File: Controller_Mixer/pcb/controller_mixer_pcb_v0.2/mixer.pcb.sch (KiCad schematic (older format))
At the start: 78 parts, among them J1 Conn_01x03, J10 Conn_01x02, J11 Conn_01x02, J12 Conn_01x02, J13 Conn_01x02, J14 Conn_01x02, J15 Conn_01x02, J16 Conn_01x02, J2 Conn_01x03, J3 Conn_01x03, J4 Conn_01x03, J41 Conn_01x04, J42 Conn_01x04, J43 Conn_01x03, J44 Conn_01x02, J45 Conn_01x02, J46 Conn_01x02, J47 Conn_01x02, J48 Conn_01x02, J49 Conn_01x02, J5 Conn_01x03, J50 Conn_01x02, J51 Conn_01x02, J52 Conn_01x02, J53 Conn_01x02, J54 Conn_01x05, J55 Conn_01x05, J56 Conn_01x05, J57 Conn_01x05, J58 Conn_01x05, J59 Conn_01x05, J6 Conn_01x03, J7 Conn_01x03, J71 Conn_01x03, J72 Conn_01x03, J8 Conn_01x03, J9 Conn_01x02, U1 74HC4051, U3 74HC4051, U5 Teensy4.1, U8 74HC4051

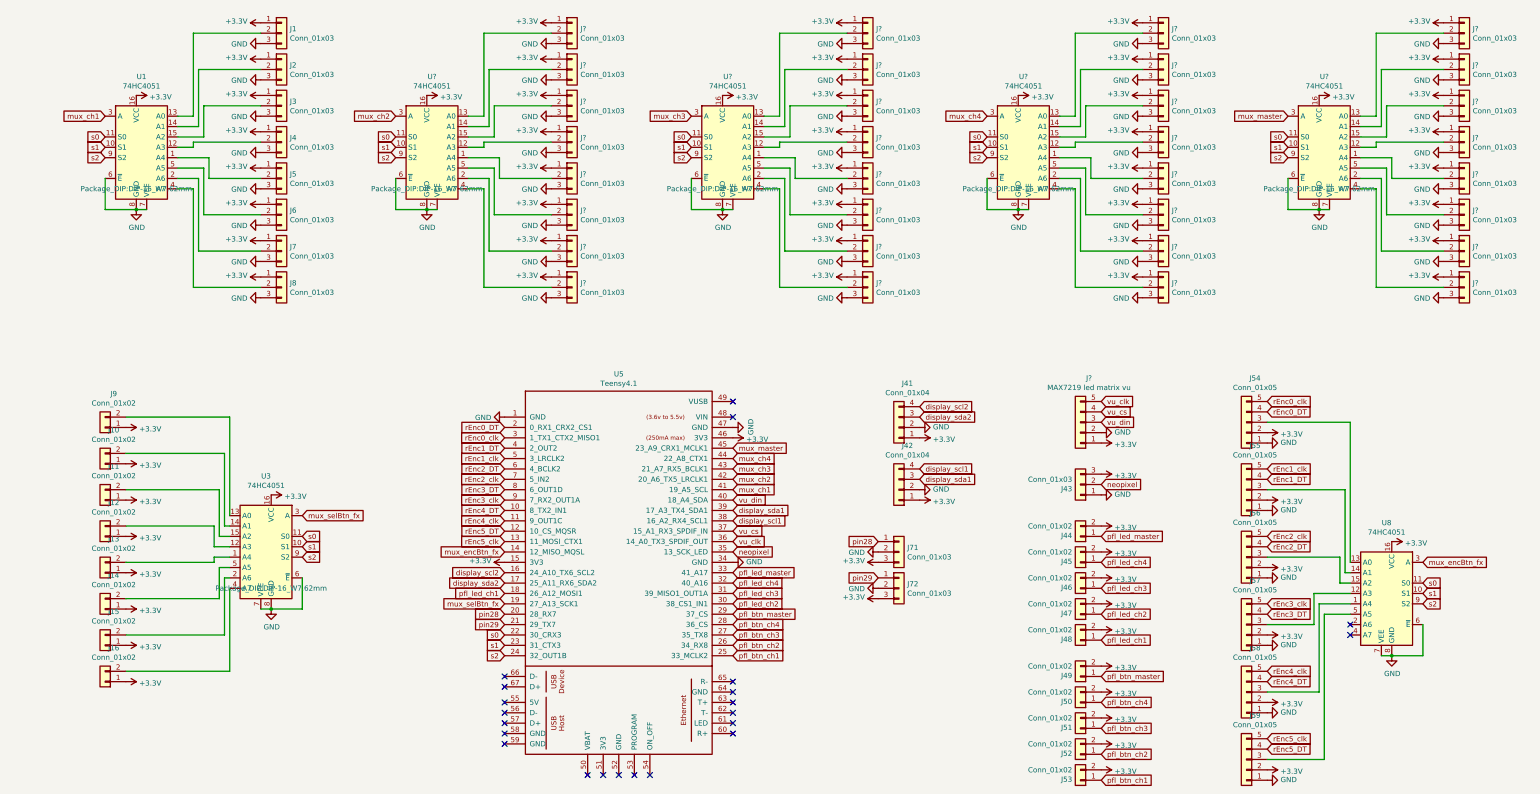
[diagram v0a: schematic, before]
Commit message: mixer pcb v0.2 ready?
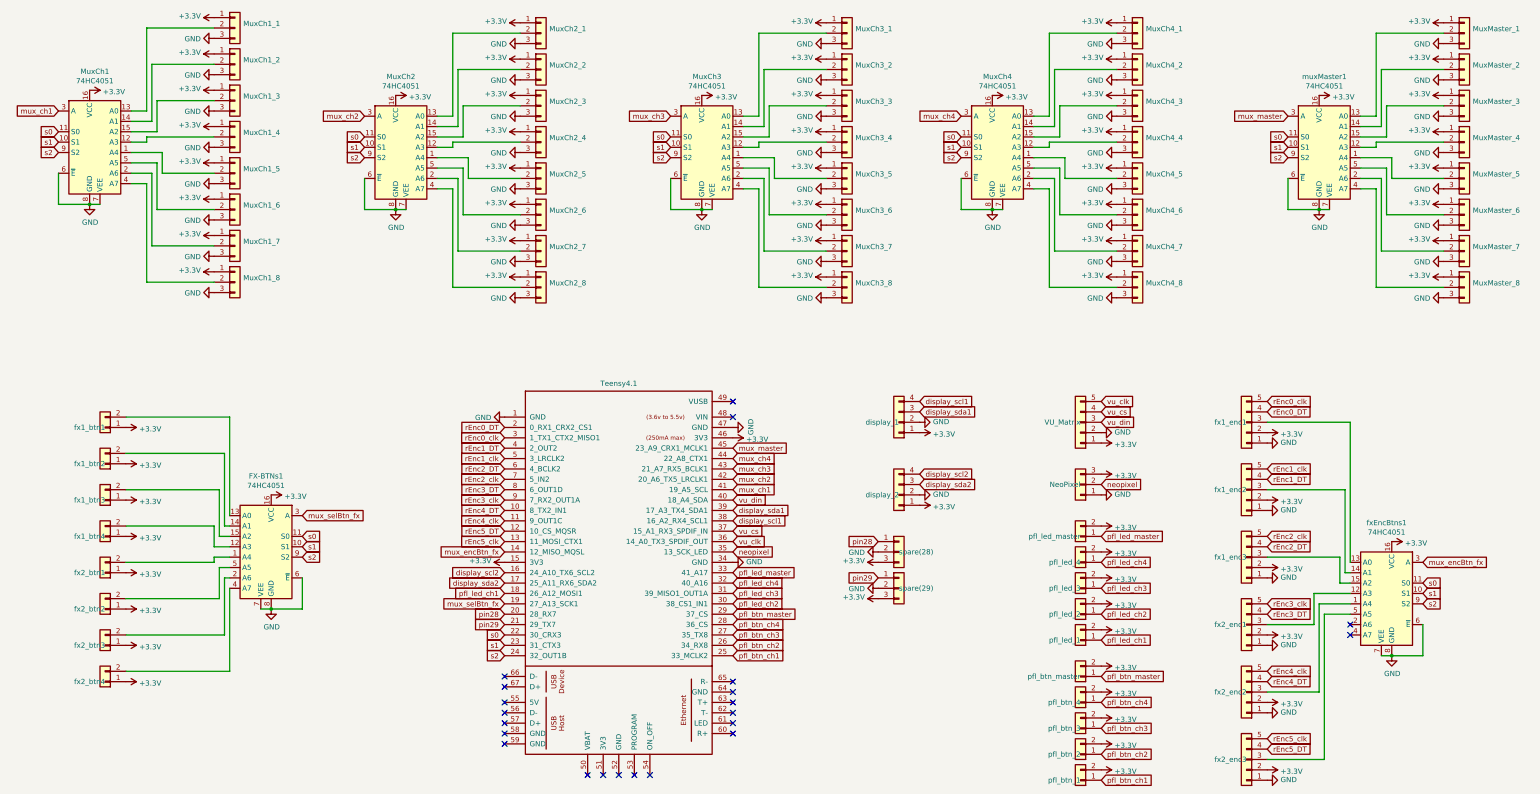
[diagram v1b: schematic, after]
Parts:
- MuxCh1_1: renamed from J?; Field4 (none) -> MuxCh1_1
- MuxCh1_2: renamed from J?; Field4 (none) -> MuxCh1_2
- MuxCh1_3: renamed from J?; Field4 (none) -> MuxCh1_3
- MuxCh1_4: renamed from J?; Field4 (none) -> MuxCh1_4
- MuxCh1_5: renamed from J?; Field4 (none) -> MuxCh1_5
- MuxCh1_6: renamed from J?; Field4 (none) -> MuxCh1_6
- MuxCh1_7: renamed from J?; Field4 (none) -> MuxCh1_7
- MuxCh1_8: renamed from J?; Field4 (none) -> MuxCh1_8
- MuxCh2_1: renamed from J?; Field4 (none) -> MuxCh2_1
- MuxCh2_2: renamed from J?; Field4 (none) -> MuxCh2_2
- MuxCh2_3: renamed from J?; Field4 (none) -> MuxCh2_3
- MuxCh2_4: renamed from J?; Field4 (none) -> MuxCh2_4
- MuxCh2_5: renamed from J?; Field4 (none) -> MuxCh2_5
- MuxCh2_6: renamed from J?; Field4 (none) -> MuxCh2_6
- MuxCh2_7: renamed from J?; Field4 (none) -> MuxCh2_7
- MuxCh2_8: renamed from J?; Field4 (none) -> MuxCh2_8
- MuxCh3_1: renamed from J1; Field4 (none) -> MuxCh3_1
- MuxCh3_2: renamed from J2; Field4 (none) -> MuxCh3_2
- MuxCh3_3: renamed from J3; Field4 (none) -> MuxCh3_3
- MuxCh3_4: renamed from J4; Field4 (none) -> MuxCh3_4
- MuxCh3_5: renamed from J5; Field4 (none) -> MuxCh3_5
- MuxCh3_6: renamed from J6; Field4 (none) -> MuxCh3_6
- MuxCh3_7: renamed from J7; Field4 (none) -> MuxCh3_7
- MuxCh3_8: renamed from J8; Field4 (none) -> MuxCh3_8
- MuxCh4_1: renamed from J?; Field4 (none) -> MuxCh4_1
- MuxCh4_2: renamed from J?; Field4 (none) -> MuxCh4_2
- MuxCh4_3: renamed from J?; Field4 (none) -> MuxCh4_3
- MuxCh4_4: renamed from J?; Field4 (none) -> MuxCh4_4
- MuxCh4_5: renamed from J?; Field4 (none) -> MuxCh4_5
- MuxCh4_6: renamed from J?; Field4 (none) -> MuxCh4_6
- MuxCh4_7: renamed from J?; Field4 (none) -> MuxCh4_7
- MuxCh4_8: renamed from J?; Field4 (none) -> MuxCh4_8
- MuxMaster_1: renamed from J?; Field4 (none) -> MuxMaster_1
- MuxMaster_2: renamed from J?; Field4 (none) -> MuxMaster_2
- MuxMaster_3: renamed from J?; Field4 (none) -> MuxMaster_3
- MuxMaster_4: renamed from J?; Field4 (none) -> MuxMaster_4
- MuxMaster_5: renamed from J?; Field4 (none) -> MuxMaster_5
- MuxMaster_6: renamed from J?; Field4 (none) -> MuxMaster_6
- MuxMaster_7: renamed from J?; Field4 (none) -> MuxMaster_7
- MuxMaster_8: renamed from J?; Field4 (none) -> MuxMaster_8
- NeoPixel1: renamed from J43; Field4 (none) -> NeoPixel
- VU_Matrix1: renamed from J?; footprint (none) -> Connector_JST:JST_XH_B5B-XH-A_1x05_P2.50mm_Vertical; Field4 (none) -> VU_Matrix
- display_1: renamed from J42; Field4 (none) -> display_1
- display_2: renamed from J41; Field4 (none) -> display_2
- fx1_btn1: renamed from J9; Field4 (none) -> fx1_btn1
- fx1_btn2: renamed from J10; Field4 (none) -> fx1_btn2
- fx1_btn3: renamed from J11; Field4 (none) -> fx1_btn3
- fx1_btn4: renamed from J12; Field4 (none) -> fx1_btn4
- fx1_enc1: renamed from J54; Field4 (none) -> fx1_enc1
- fx1_enc2: renamed from J55; Field4 (none) -> fx1_enc2
- fx1_enc3: renamed from J56; Field4 (none) -> fx1_enc3
- fx2_btn1: renamed from J13; Field4 (none) -> fx2_btn1
- fx2_btn2: renamed from J14; Field4 (none) -> fx2_btn2
- fx2_btn3: renamed from J15; Field4 (none) -> fx2_btn3
- fx2_btn4: renamed from J16; Field4 (none) -> fx2_btn4
- fx2_enc1: renamed from J57; Field4 (none) -> fx2_enc1
- fx2_enc2: renamed from J58; Field4 (none) -> fx2_enc2
- fx2_enc3: renamed from J59; Field4 (none) -> fx2_enc3
- pfl_btn_1: renamed from J53; Field4 (none) -> pfl_btn_1
- pfl_btn_2: renamed from J52; Field4 (none) -> pfl_btn_2
- pfl_btn_3: renamed from J51; Field4 (none) -> pfl_btn_3
- pfl_btn_4: renamed from J50; Field4 (none) -> pfl_btn_4
- pfl_btn_master1: renamed from J49; Field4 (none) -> pfl_btn_master
- pfl_led_1: renamed from J48; Field4 (none) -> pfl_led_1
- pfl_led_2: renamed from J47; Field4 (none) -> pfl_led_2
- pfl_led_3: renamed from J46; Field4 (none) -> pfl_led_3
- pfl_led_4: renamed from J45; Field4 (none) -> pfl_led_4
- pfl_led_master1: renamed from J44; Field4 (none) -> pfl_led_master
- spare(28)1: renamed from J71; Field4 (none) -> spare(28)
- spare(29)1: renamed from J72; Field4 (none) -> spare(29)
- gave numbers to parts that had none: 4
- renumbered U3 to FX-BTNs1, U1 to MuxCh3, U8 to fxEncBtns1
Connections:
- net mux_ch1: now also MuxCh1.3 (A); no longer MuxCh3.3 (A)
- net mux_ch2: now also MuxCh2.3 (A); no longer MuxCh4.3 (A)
- net mux_ch3: now also MuxCh3.3 (A); no longer MuxCh2.3 (A)
- net mux_ch4: now also MuxCh4.3 (A); no longer MuxCh1.3 (A)
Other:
- moved on the sheet: MuxCh1, MuxCh1_1, MuxCh1_2, MuxCh1_3, MuxCh1_4, MuxCh1_5, MuxCh1_6, MuxCh1_7, MuxCh1_8, MuxCh2, MuxCh2_1, MuxCh2_2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
